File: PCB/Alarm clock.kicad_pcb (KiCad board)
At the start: 4 copper layers, 4 parts, among them J1 TFT, J2 RTC, SW1 SW_MEC_5G, U1 ESP32-C3_SUPERMINI

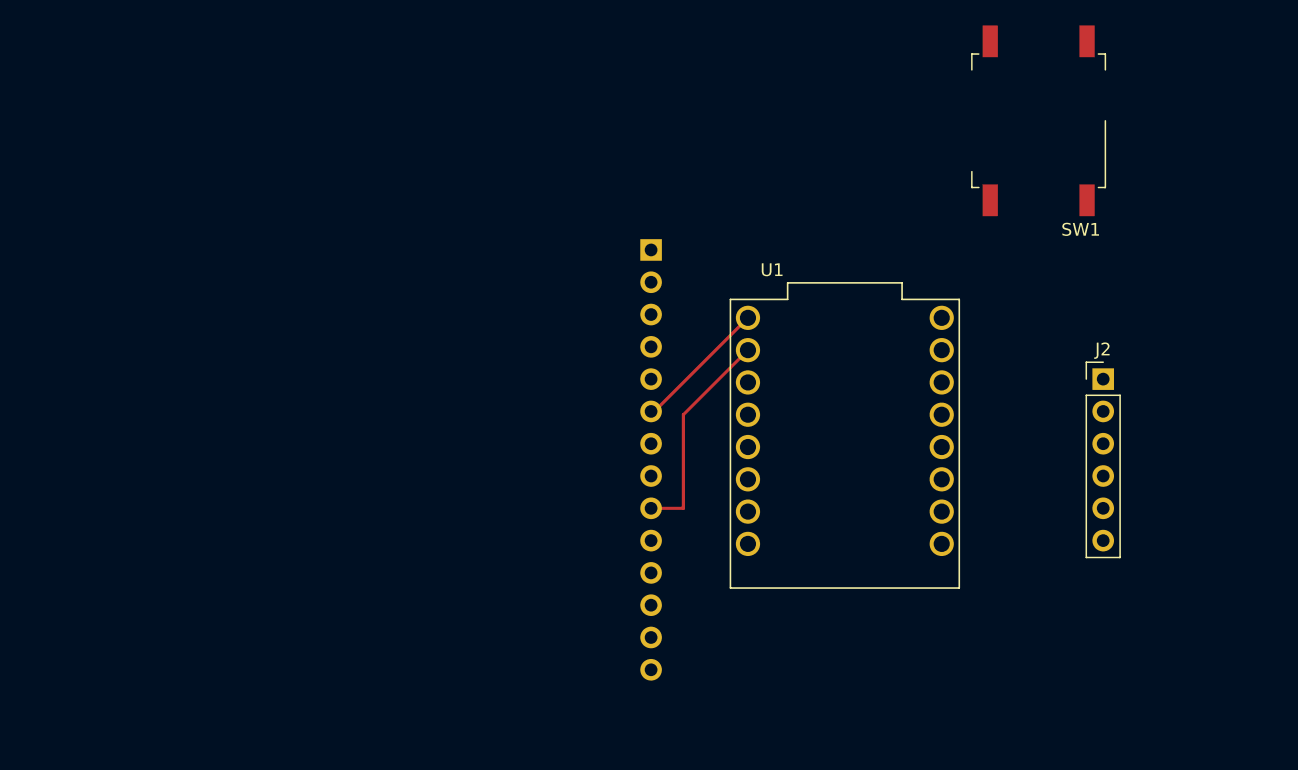
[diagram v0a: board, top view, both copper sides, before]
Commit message: PCB Update
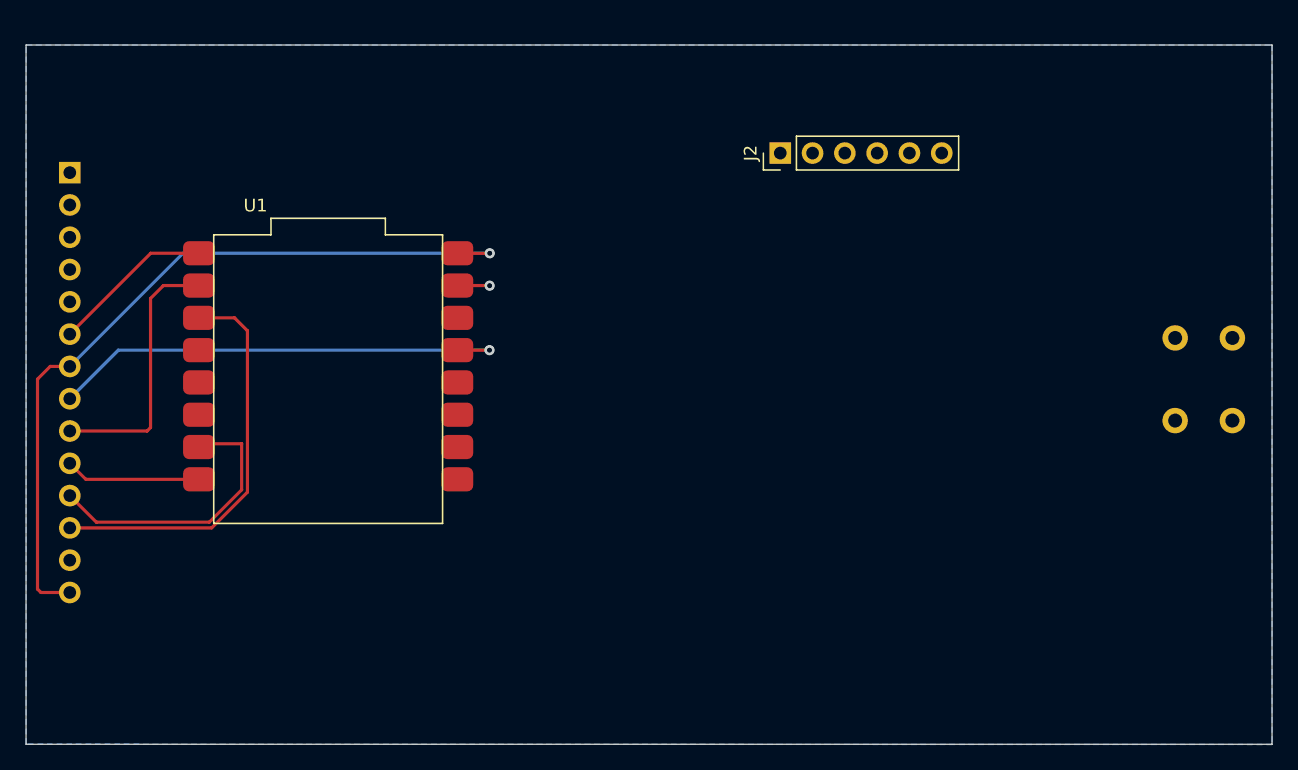
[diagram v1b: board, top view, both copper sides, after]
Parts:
- SW1: value SW_MEC_5G -> SW_Push; footprint Button_Switch_SMD:SW_MEC_5GSH9 -> Button_Switch_THT:SW_PUSH_6mm; moved to B.Cu
- moved J1 46.1 mm to (91.4, 65.0)
- moved U1 41.0 mm to (111.8, 81.3)
- moved J2 31.0 mm to (147.3, 63.5), turned to 90 degrees
- moved SW1 28.1 mm to (182.9, 84.5), turned to 90 degrees
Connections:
- SW1 pad 1: Net-(SW1-Pad1) -> Net-(U1-Pad10)
- SW1 pad 2: Net-(SW1-Pad1) -> GND
- U1 pad 10: Net-(SW1-Pad1) -> Net-(U1-Pad10)
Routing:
- net +5V: track 0.00 -> 61.4 mm, vias 0 -> 1
- net Net-(J1-Pad8): track 0.00 -> 37.1 mm, vias 0 -> 1
- net Net-(J1-Pad12): track 0.00 -> 32.1 mm
- net Net-(J1-Pad11): track 0.00 -> 22.5 mm
- net Net-(J1-Pad10): track 0.00 -> 10.7 mm
- net Net-(J1-Pad9): track 17.1 -> 20.9 mm
- net GND: track 0.00 -> 2.80 mm, vias 0 -> 1
- net Net-(J1-Pad6): track 10.7 -> 12.8 mm
- added copper zone on B.Cu, net GND
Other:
- board outline added: 98 x 55 mm
